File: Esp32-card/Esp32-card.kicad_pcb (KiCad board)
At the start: 2 copper layers, 60 x 80 mm, 6 parts, among them J1 Conn_01x12_Pin, U1 74HC595, U2 74HC595, U3 L298N, U4 74HC4051

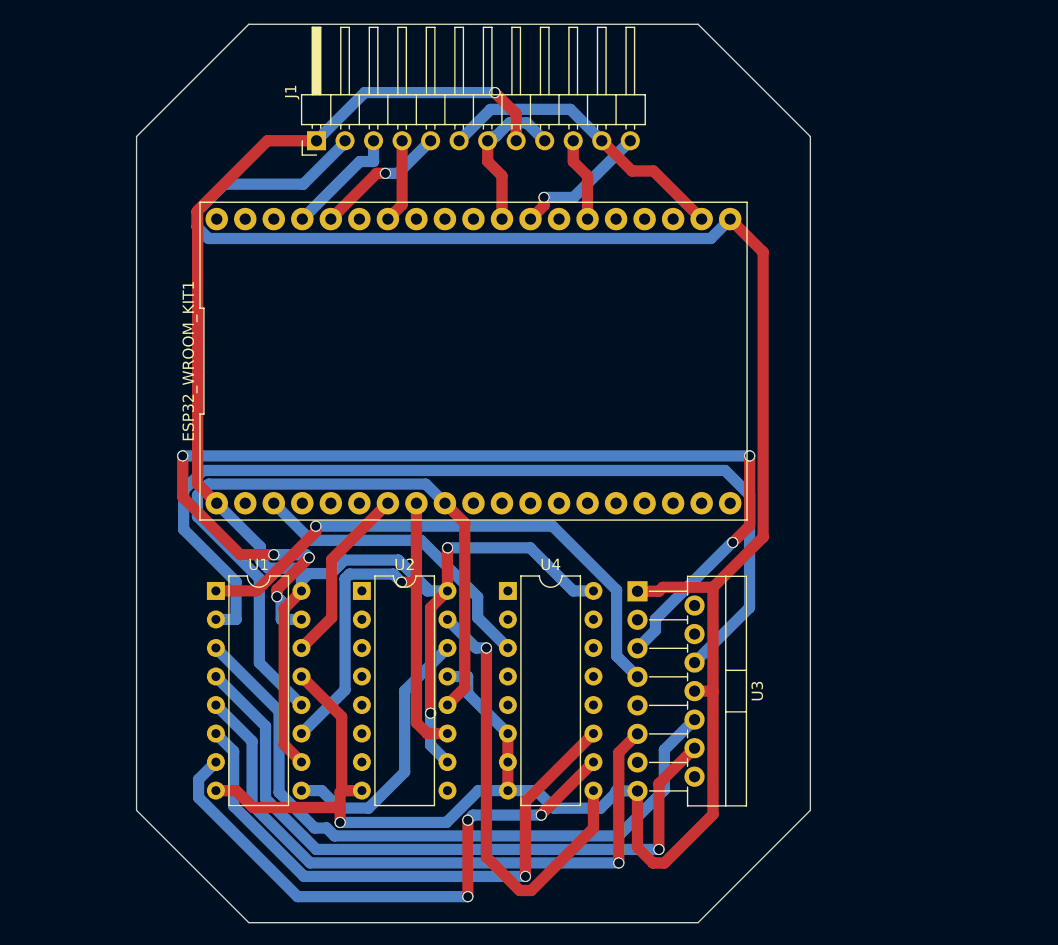
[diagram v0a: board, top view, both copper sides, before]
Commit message: Alimentation
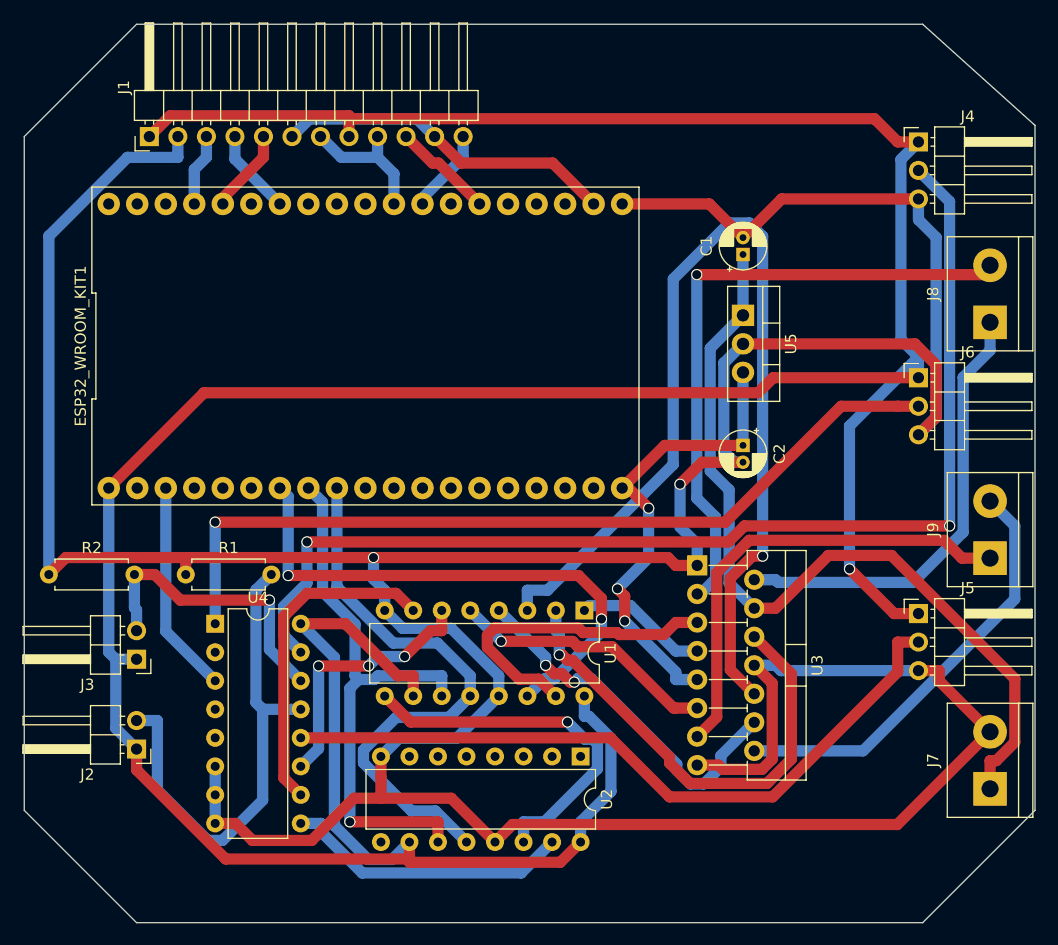
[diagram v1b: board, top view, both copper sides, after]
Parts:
- added C1: C, Capacitor_THT:CP_Radial_D4.0mm_P1.50mm, F.Cu at (174.0, 70.5)
- added C2: C, Capacitor_THT:CP_Radial_D4.0mm_P1.50mm, F.Cu at (174.0, 87.5)
- added J2: Conn_01x02_Pin, Connector_PinHeader_2.54mm:PinHeader_1x02_P2.54mm_Horizontal, F.Cu at (120.0, 114.5)
- added J3: Conn_01x02_Pin, Connector_PinHeader_2.54mm:PinHeader_1x02_P2.54mm_Horizontal, F.Cu at (120.0, 106.5)
- added J4: Conn_01x03_Pin, Connector_PinHeader_2.54mm:PinHeader_1x03_P2.54mm_Horizontal, F.Cu at (189.6, 60.5)
- added J5: Conn_01x03_Pin, Connector_PinHeader_2.54mm:PinHeader_1x03_P2.54mm_Horizontal, F.Cu at (189.6, 102.5)
- added J6: Conn_01x03_Pin, Connector_PinHeader_2.54mm:PinHeader_1x03_P2.54mm_Horizontal, F.Cu at (189.6, 81.5)
- added J7: Conn_01x02_Socket, TerminalBlock:TerminalBlock_bornier-2_P5.08mm, F.Cu at (196.0, 118.1)
- added J8: Conn_01x02_Socket, TerminalBlock:TerminalBlock_bornier-2_P5.08mm, F.Cu at (196.0, 76.5)
- added J9: Conn_01x02_Socket, TerminalBlock:TerminalBlock_bornier-2_P5.08mm, F.Cu at (196.0, 97.5)
- added R1: R, Resistor_THT:R_Axial_DIN0207_L6.3mm_D2.5mm_P7.62mm_Horizontal, F.Cu at (124.4, 99.0)
- added R2: R, Resistor_THT:R_Axial_DIN0207_L6.3mm_D2.5mm_P7.62mm_Horizontal, F.Cu at (112.2, 99.0)
- added U5: L7805, Package_TO_SOT_THT:TO-220-3_Vertical, F.Cu at (174.0, 75.9)
- moved U1 32.9 mm to (159.9, 102.2), turned to -90 degrees
- moved U4 26.2 mm to (127.0, 103.4)
- moved U2 24.4 mm to (159.5, 115.2), turned to -90 degrees
- moved J1 14.9 mm to (121.1, 60.0)
- moved ESP32_WROOM_KIT1 9.71 mm to (140.4, 78.7)
- moved U3 5.79 mm to (169.9, 98.2)
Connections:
- ESP32_WROOM_KIT1 pad 19: unconnected-(ESP32_WROOM_KIT1-5V-Pad19) -> 5v
- U3 pad 13: unconnected-(U3-OUT3-Pad13) -> Net-(J9-Pin_1)
- U3 pad 14: unconnected-(U3-OUT4-Pad14) -> Net-(J9-Pin_2)
- U3 pad 2: unconnected-(U3-OUT1-Pad2) -> Net-(J8-Pin_1)
- U3 pad 3: unconnected-(U3-OUT2-Pad3) -> Net-(J8-Pin_2)
- U4 pad 1: unconnected-(U4-A4-Pad1) -> Capteur_Hall_3
- U4 pad 12: unconnected-(U4-A3-Pad12) -> Capteur_Hall_2
- U4 pad 13: unconnected-(U4-A0-Pad13) -> Capteur_Flexion_1
- U4 pad 14: unconnected-(U4-A1-Pad14) -> Capteur_Flexion_2
- U4 pad 15: unconnected-(U4-A2-Pad15) -> Capteur_Hall_1
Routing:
- net 3v3: track 141.6 -> 329.8 mm, vias 3 -> 1
- net GND: track 215.1 -> 367.5 mm, vias 1 -> 2
- net Capteur_Hall_1: track 0.00 -> 101.9 mm, vias 0 -> 2
- net Capteur_Hall_3: track 0.00 -> 75.9 mm, vias 0 -> 1
- net Power supply: track 0.00 -> 75.1 mm
- net M1_Pin_Dir1: track 97.6 -> 28.6 mm, vias 6 -> 0
- net Capteur_Hall_2: track 0.00 -> 64.4 mm
- net Net-(J8-Pin_2): track 0.00 -> 56.4 mm, vias 0 -> 1
- net Capteur_Flexion_1: track 0.00 -> 45.1 mm
- net 5v: track 0.00 -> 42.4 mm, vias 0 -> 3
- net Net-(J9-Pin_1): track 0.00 -> 41.5 mm
- net M1_Pin_EN: track 84.2 -> 42.9 mm, vias 0 -> 1
- net Net-(J8-Pin_1): track 0.00 -> 40.2 mm
- net Net-(J9-Pin_2): track 0.00 -> 38.4 mm
- net M1_Pin_Dir2: track 49.2 -> 11.9 mm, vias 1 -> 0
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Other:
- board size 60 x 80 mm -> 90 x 80 mm

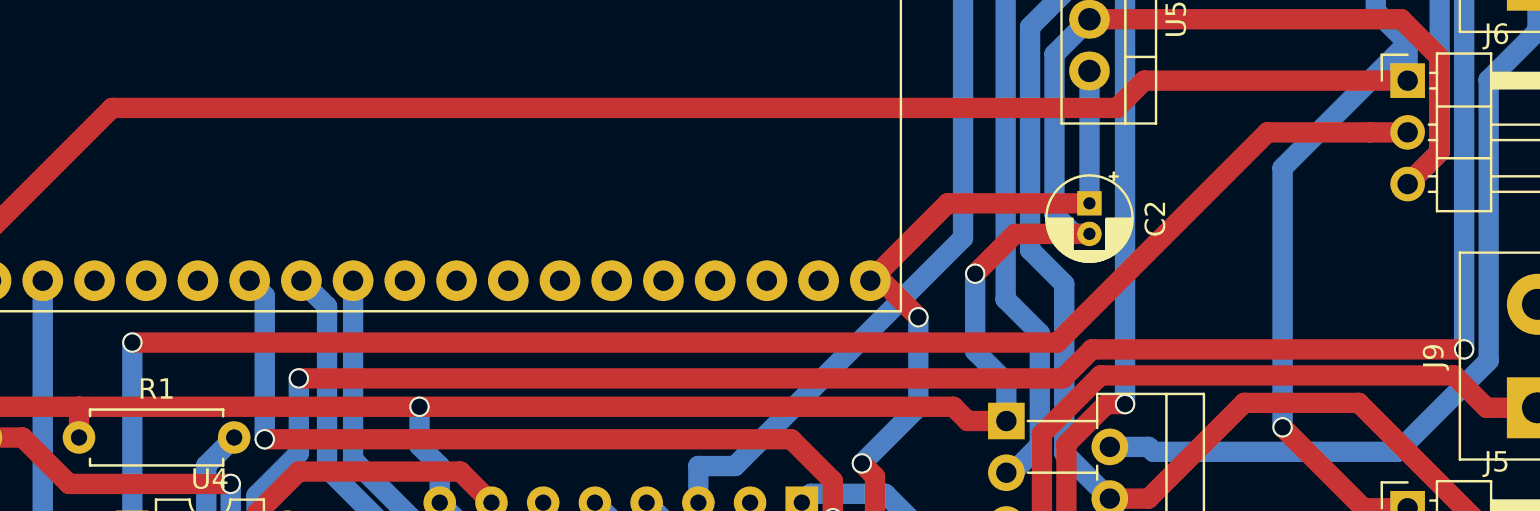
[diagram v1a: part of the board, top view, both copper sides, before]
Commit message: .
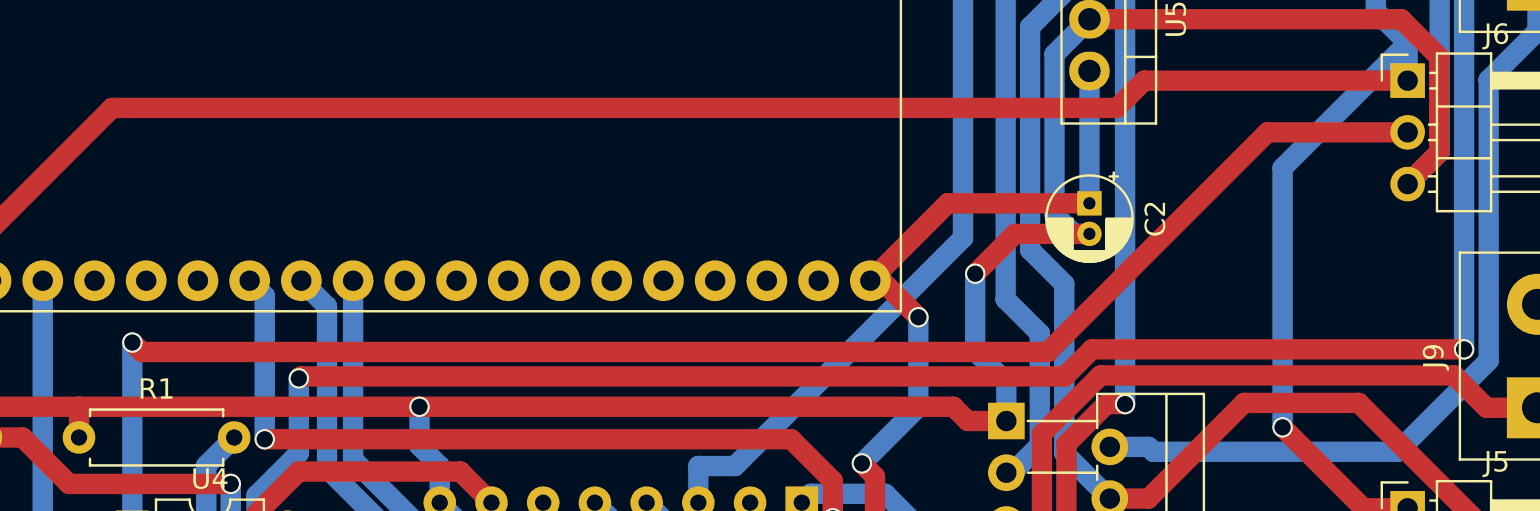
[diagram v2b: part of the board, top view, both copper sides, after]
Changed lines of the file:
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@@
-	)
-	(segment
-		(start 172.6994 96.0966)
-		(end 174.1251 94.6709)
-		(width 1)
-		(layer "F.Cu")
-		(net 65)
 	)
 	(segment
 		(start 135.1754 96.0966)
-		(end 172.6994 96.0966)
+		(end 135.272 96)
 		(width 1)
 		(layer "F.Cu")
@@
 		(start 174.1251 94.6709)
 		(end 192.3996 94.6709)
+		(width 1)
+		(layer "F.Cu")
+		(net 65)
+	)
+	(segment
+		(start 172.796 96)
+		(end 174.1251 94.6709)
+		(width 1)
+		(layer "F.Cu")
+		(net 65)
+	)
+	(segment
+		(start 135.272 96)
+		(end 172.796 96)
 		(width 1)
 		(layer "F.Cu")
@@
 	)
 	(segment
-		(start 189.625 84.015)
-		(end 187.775 84.015)
+		(start 127.4631 94.8)
+		(end 127 94.3369)
+		(width 1)
+		(layer "F.Cu")
+		(net 69)
+	)
+	(segment
+		(start 171.9564 94.8)
+		(end 127.4631 94.8)
 		(width 1)
 		(layer "F.Cu")
@@
 	(segment
 		(start 182.7414 84.015)
-		(end 172.4195 94.3369)
+		(end 171.9564 94.8)
 		(width 1)
 		(layer "F.Cu")
@@
 	)
 	(segment
-		(start 187.775 84.015)
+		(start 189.625 84.015)
 		(end 182.7414 84.015)
 		(width 1)
 		(layer "F.Cu")
-		(net 69)
-	)
-	(segment
-		(start 172.4195 94.3369)
-		(end 127 94.3369)
-		(width 1)
-		(layer "F.Cu")
